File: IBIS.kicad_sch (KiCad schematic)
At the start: 29 parts, among them J1 Screw_Terminal_01x06, J1 USB_B_Mini, T1 BC337, T2 BC556, U1 CH340G, U2 MAX232, X1 12MHz

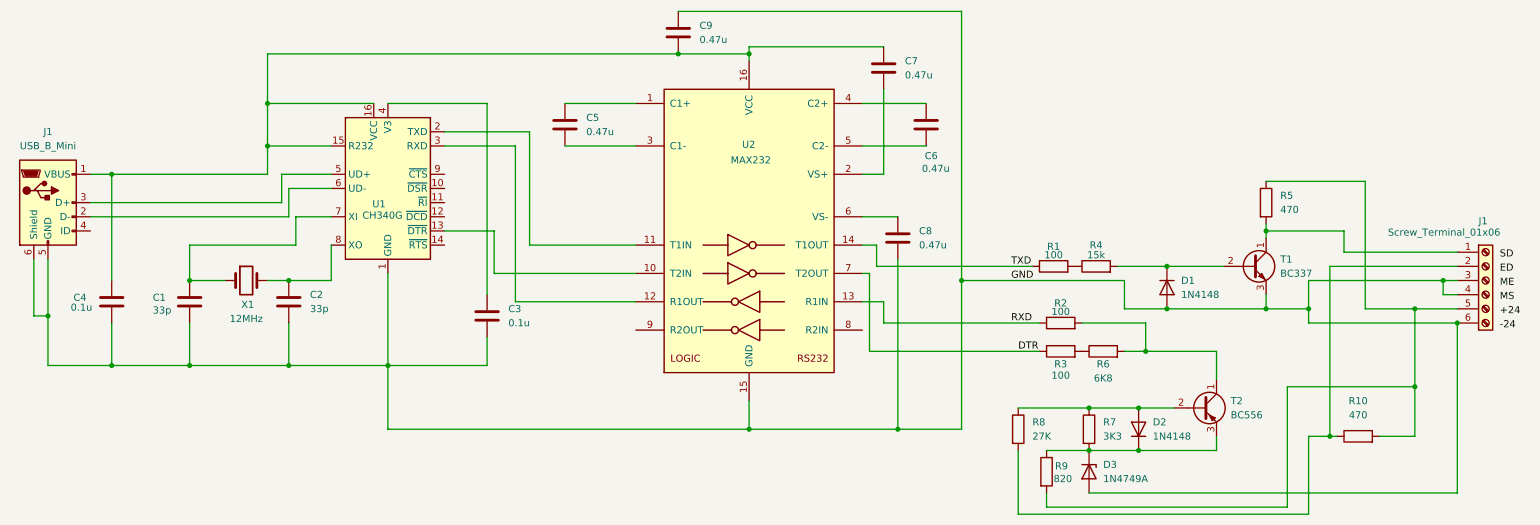
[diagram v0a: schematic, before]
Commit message: PCB design
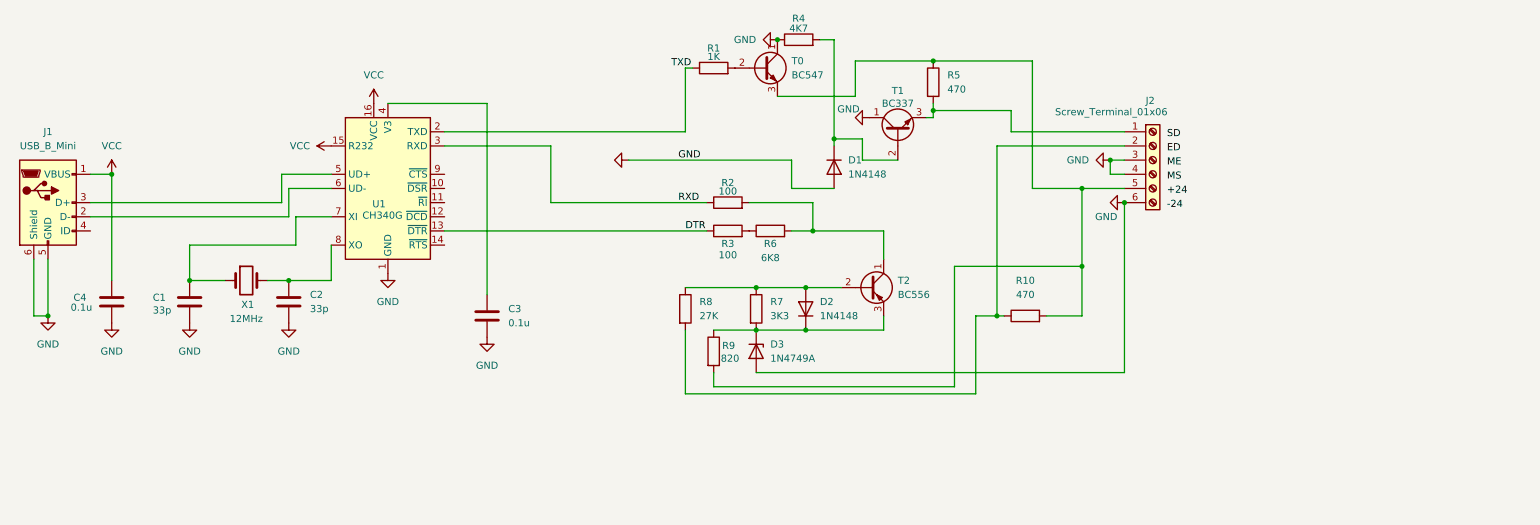
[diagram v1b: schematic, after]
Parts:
- removed C5, C6, C7, C8, C9: 0.47u, symbol Device:C
- removed U2: MAX232, symbol Interface_UART:MAX232
- added T0: BC547, Package_TO_SOT_THT:TO-92_Inline, symbol Transistor_BJT:BC547
- C1, C2, C3, C4: footprint (none) -> Capacitor_THT:C_Disc_D7.5mm_W5.0mm_P5.00mm
- D1, D2: footprint (none) -> Diode_THT:D_DO-35_SOD27_P10.16mm_Horizontal
- J1: footprint (none) -> Connector_USB:USB_Mini-B_Wuerth_65100516121_Horizontal
- J2: renamed from J1; footprint (none) -> TerminalBlock_WAGO:TerminalBlock_WAGO_233-506_2x06_P2.54mm
- R1: value 100 -> 1K; footprint (none) -> Resistor_THT:R_Axial_DIN0207_L6.3mm_D2.5mm_P10.16mm_Horizontal
- R10, R2, R3, R5, R6, R7, R8, R9: footprint (none) -> Resistor_THT:R_Axial_DIN0207_L6.3mm_D2.5mm_P10.16mm_Horizontal
- R4: value 15k -> 4K7; footprint (none) -> Resistor_THT:R_Axial_DIN0207_L6.3mm_D2.5mm_P10.16mm_Horizontal
- X1: footprint (none) -> Crystal:Crystal_HC49-4H_Vertical
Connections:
- net DTR: now also U1.13 (~{DTR})
- net GND: now also R4.1, T1.1 (C), T0.1 (C); no longer T1.3 (E)
- net RXD: now also U1.3 (RXD)
- net TXD: no longer R1.1
- net VCC: now reaches C4.1, J1.1 (VBUS), U1.15 (R232), U1.16 (VCC)
- net at U1.2 (TXD): now also R1.1
- net at J2.1 (Pin_1), R5.2: now also T1.3 (E); no longer T1.1 (C)
- net at J2.5 (Pin_5), R10.2, R5.1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: now also T0.3 (E)
- net at R1.2: now also T0.2 (B); no longer R4.1
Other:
- moved on the sheet: D1, D2, D3, J2, R1, R10, R2, R3, R4, R5, R6, R7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
